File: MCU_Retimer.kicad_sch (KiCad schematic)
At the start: 39 parts, among them J10 SWD, J11 UART, J12 I2C1, Q16 AO3401A, Q17 2N7002W

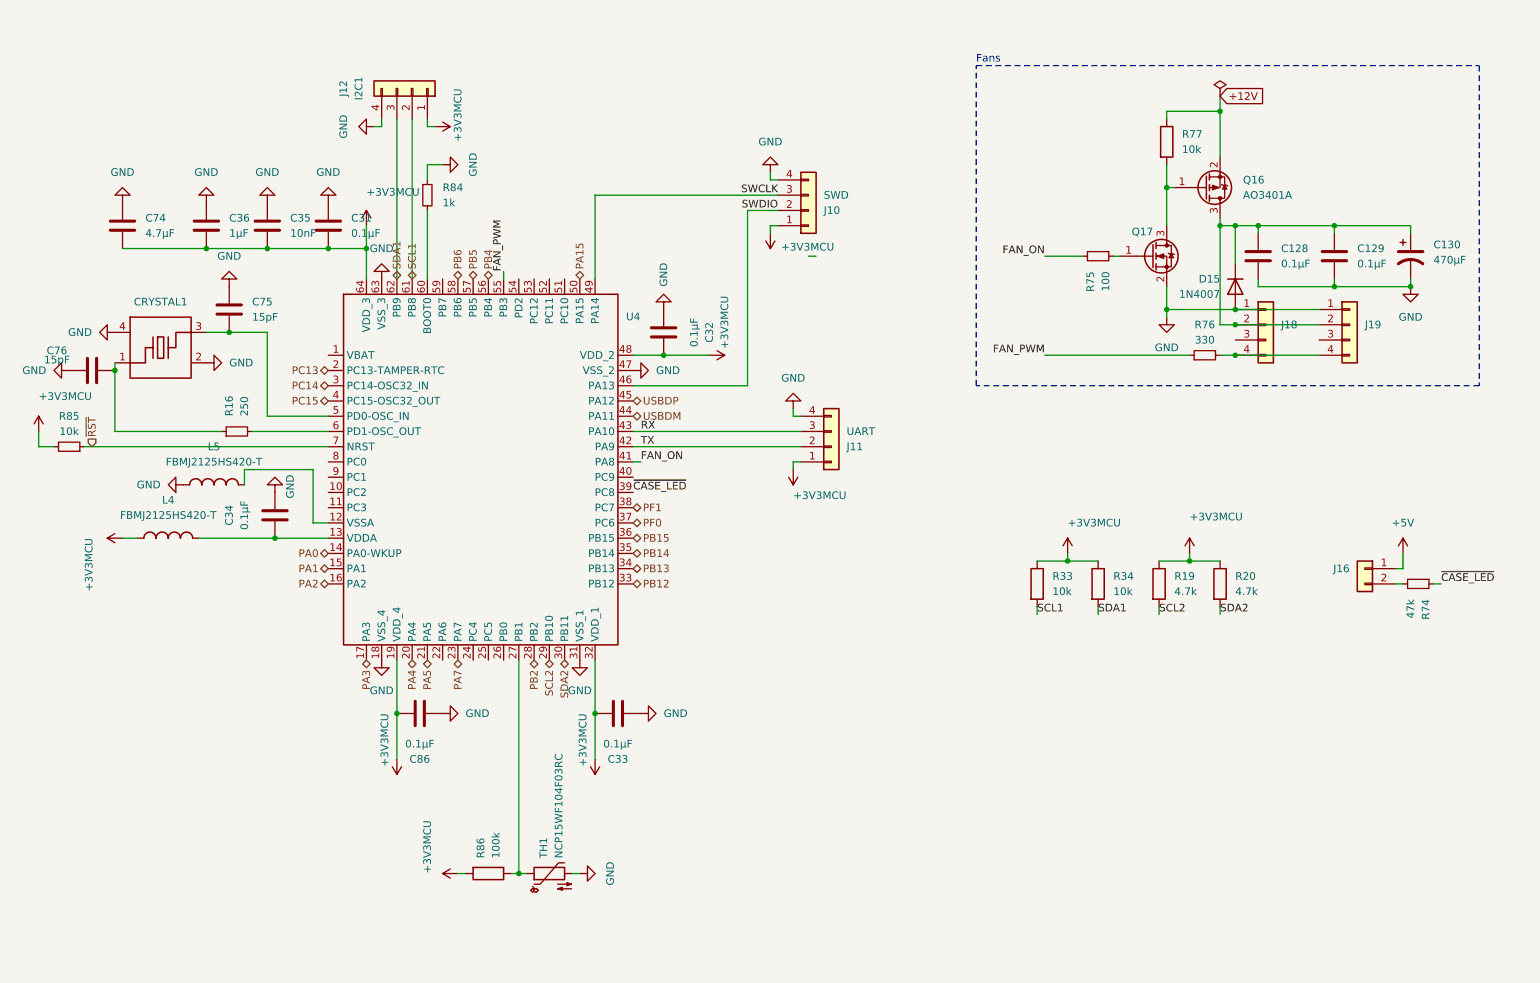
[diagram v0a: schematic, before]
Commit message: eeeeeeeee
eeeeeeeee
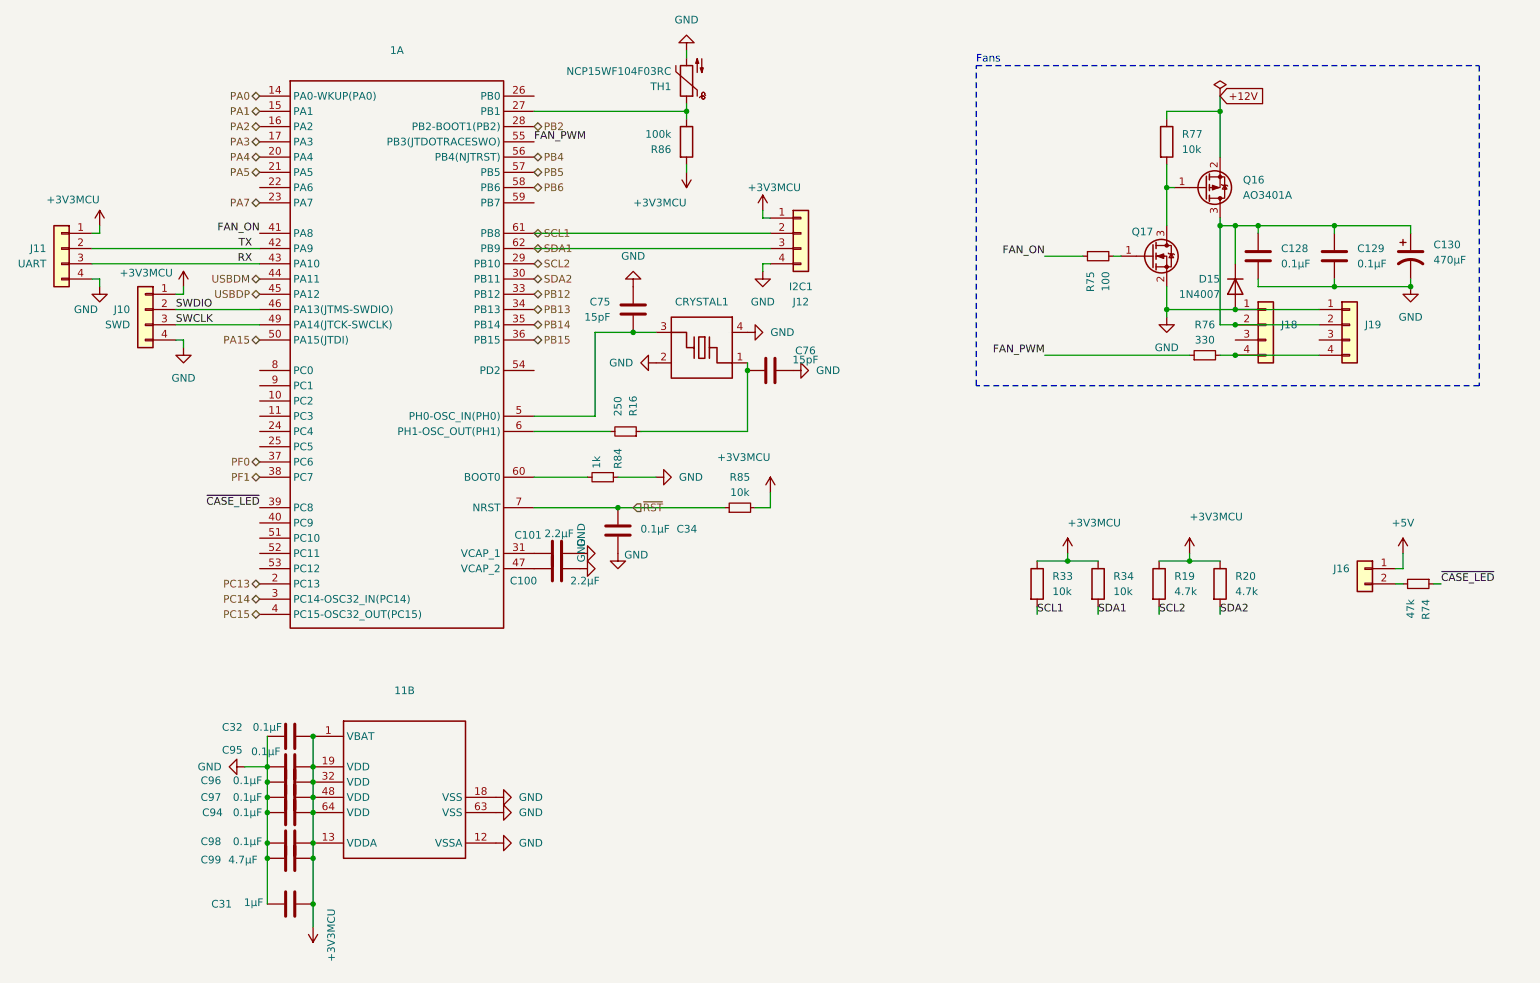
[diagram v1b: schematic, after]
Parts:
- removed C33, C86: 0.1µF, Capacitor_SMD:C_0402_1005Metric, symbol Device:C
- removed C35: 10nF, Capacitor_SMD:C_0402_1005Metric, symbol Device:C
- removed C36: 1µF, Capacitor_SMD:C_0402_1005Metric, symbol Device:C
- removed C74: 4.7µF, Capacitor_SMD:C_0402_1005Metric, symbol Device:C
- removed L4, L5: FBMJ2125HS420-T, FBMJ2125HS420-T:L0805, symbol FBMJ2125HS420-T:FBMJ2125HS420-T
- removed U4: ~, STM32F103RCT6:LQFP-64_L10.0-W10.0-P0.50-LS12.0-BL, symbol STM32F103RCT6:STM32F103RCT6
- added 1, 11: ~, STM32F405RGT6:LQFP-64_L10.0-W10.0-P0.50-LS12.0-BL, symbol STM32F405RGT6:STM32F405RGT6
- added C100, C101: 2.2µF, Capacitor_SMD:C_0603_1608Metric, symbol Device:C
- added C94, C95, C96, C97, C98: 0.1µF, Capacitor_SMD:C_0402_1005Metric, symbol Device:C
- added C99: 4.7µF, Capacitor_SMD:C_0402_1005Metric, symbol Device:C
- C31: value 0.1µF -> 1µF; LCSC C307331 -> C1592; Part_Number CL05B104KB54PNC -> CL10A105KO8NNNC
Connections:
- net +3V3MCU: now also C31.1, 11.1 (VBAT), 11.13 (VDDA), 11.19 (VDD), 11.32 (VDD), 11.48 (VDD), 11.64 (VDD), C94.2, C95.2, C96.2, C97.2, C98.2, C99.1; no longer C31.2
- net FAN_ON: now also 1.41 (PA8)
- net FAN_PWM: now also 1.55 (PB3(JTDOTRACESWO))
- net GND: now also C31.2, C34.2, 11.12 (VSSA), 11.18 (VSS), 11.63 (VSS), C100.1, C101.1, C94.1, C95.1, C96.1, C97.1, C98.1, C99.2; no longer C31.1, C34.1
- net PA0: now also 1.14 (PA0-WKUP(PA0))
- net PA1: now also 1.15 (PA1)
- net PA15: now also 1.50 (PA15(JTDI))
- net PA2: now also 1.16 (PA2)
- net PA3: now also 1.17 (PA3)
- net PA4: now also 1.20 (PA4)
- net PA5: now also 1.21 (PA5)
- net PA7: now also 1.23 (PA7)
- net PB12: now also 1.33 (PB12)
- net PB13: now also 1.34 (PB13)
- net PB14: now also 1.35 (PB14)
- net PB15: now also 1.36 (PB15)
- net PB2: now also 1.28 (PB2-BOOT1(PB2))
- net PB4: now also 1.56 (PB4(NJTRST))
- net PB5: now also 1.57 (PB5)
- net PB6: now also 1.58 (PB6)
- net PC13: now also 1.2 (PC13)
- net PC14: now also 1.3 (PC14-OSC32_IN(PC14))
- net PC15: now also 1.4 (PC15-OSC32_OUT(PC15))
- net PF0: now also 1.37 (PC6)
- net PF1: now also 1.38 (PC7)
- net RX: now also 1.43 (PA10)
- net SCL1: now also 1.61 (PB8)
- net SCL2: now also 1.29 (PB10)
- net SDA1: now also 1.62 (PB9)
- net SDA2: now also 1.30 (PB11)
- net SWCLK: now also 1.49 (PA14(JTCK-SWCLK))
- net SWDIO: now also 1.46 (PA13(JTMS-SWDIO))
- net TX: now also 1.42 (PA9)
- net USBDM: now also 1.44 (PA11)
- net USBDP: now also 1.45 (PA12)
- net ~{CASE_LED}: now also 1.39 (PC8)
- net ~{RST}: now also C34.1, 1.7 (NRST)
- net at C75.2, CRYSTAL1.3: now also 1.5 (PH0-OSC_IN(PH0))
- net at R16.2: now also 1.6 (PH1-OSC_OUT(PH1))
- net at R86.1, TH1.1: now also 1.27 (PB1)
- net at R84.2: now also 1.60 (BOOT0)
- new net: 1.47 (VCAP_2), C100.2
- new net: 1.31 (VCAP_1), C101.2
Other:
- moved on the sheet: C75, C76, CRYSTAL1, J10, J11, J12, R16, R84, R85, R86, TH1
